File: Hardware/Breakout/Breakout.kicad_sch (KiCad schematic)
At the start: 12 parts, among them IC1 NUCLEO-G431KB, J1 Conn_Coaxial, U1 TDC7200PWR, U2 BUF602ID, U3 MAX9011EUT+T, U4 MAX7375AXR805+T

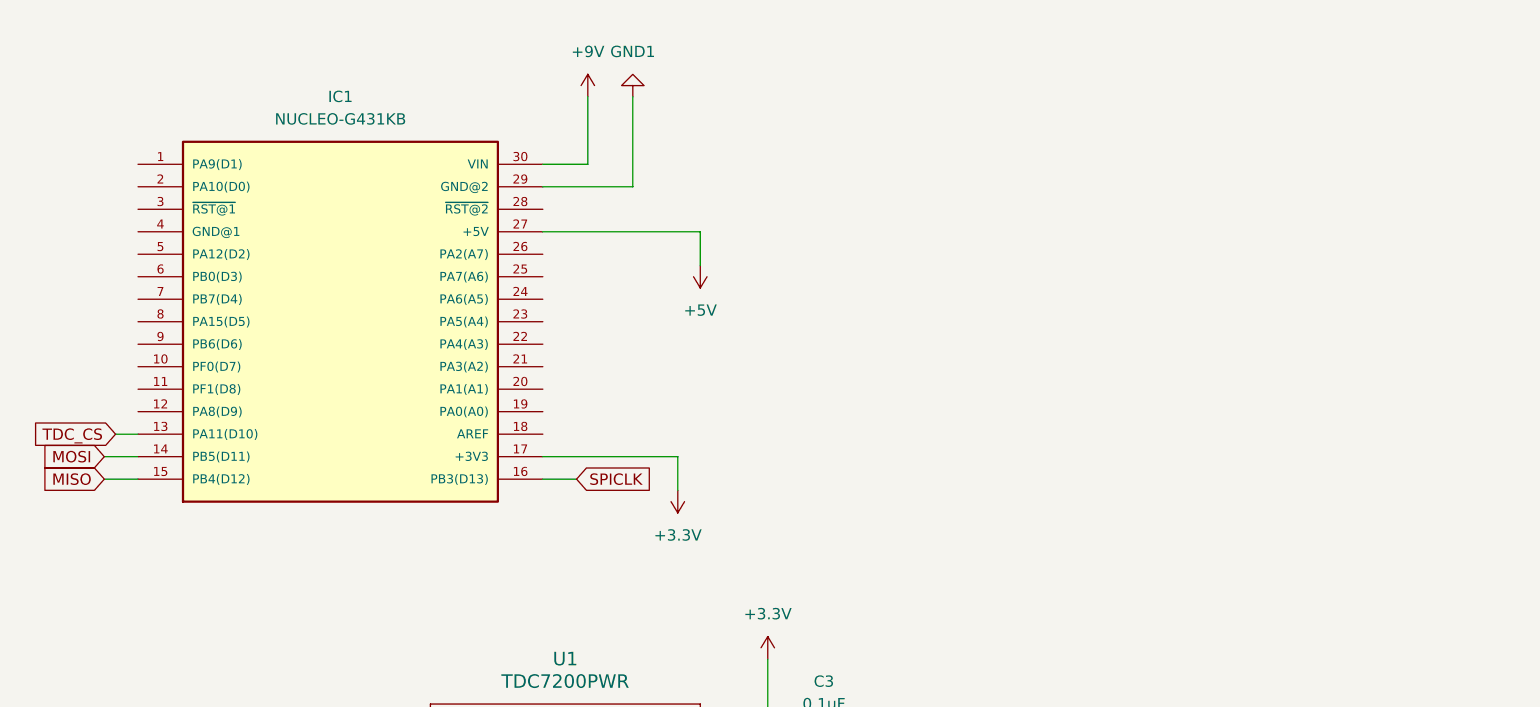
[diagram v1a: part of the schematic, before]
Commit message: Upload of hardware changes as of 6pm 06/07/2023
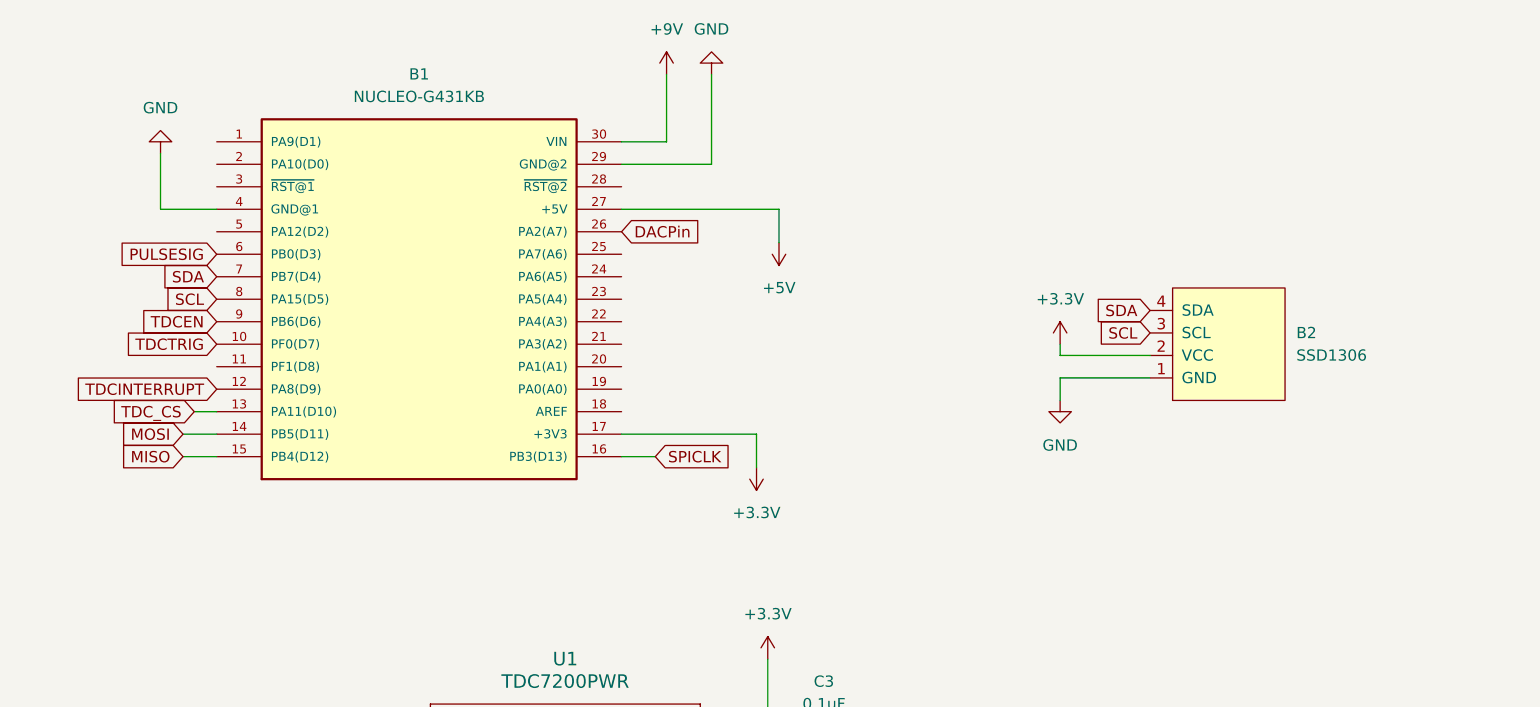
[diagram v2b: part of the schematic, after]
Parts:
- added B2: SSD1306, Library:Adafruit_SSD1306_4Pin, symbol SSD1306-128x64_OLED:SSD1306
- B1: renamed from IC1; footprint (none) -> NUCLEO-G431KB:DIPS1524W66P254L5029H1500Q30N
- C1: footprint (none) -> UWT1HH010MCL1GB:PCAP_4x5.4-ELECT_NCA-L
- C2, C3, C4, C5: footprint (none) -> 06035C104JAT2A:CAPC1608X90N
- J1: footprint (none) -> Library:0731375003_BCN_conn
- U1: footprint PW0014A_N -> TDC7200PWR:SOP65P640X120-14N
- U2: footprint D0008A_N -> BUF602ID:D0008A_N
- U3: footprint 21-0058I_MXM -> MAX9011EUT:21-0058I_MXM
- U4: footprint 21-0075D_MXM -> MAX737AXR805:21-0075D_MXM
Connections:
- net GND1 is gone; now on net GND: B1.29 (GND@2)
- net +3.3V: now also B2.2 (VCC)
- net DACPin: now also B1.26 (PA2(A7))
- net GND: now also B1.4 (GND@1), B2.1 (GND)
- net PULSESIG: now also B1.6 (PB0(D3))
- net TDCEN: now also B1.9 (PB6(D6))
- net TDCINTERRUPT: now also B1.12 (PA8(D9))
- net TDCTRIG: now also B1.10 (PF0(D7))
- net SDA: now reaches B1.7 (PB7(D4))
- net SDA: now also B2.4 (SDA)
- net SCL: now reaches B1.8 (PA15(D5))
- net SCL: now also B2.3 (SCL)
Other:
- moved on the sheet: B1
